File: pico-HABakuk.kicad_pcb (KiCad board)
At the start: 2 copper layers, 52 x 51.2 mm, 87 parts, among them J1 USB_B_Micro, J2 Ant+, J3 GPS Ant, J4 Ant-, J5 Solar, J6 Debug, J7 Super_Cap, Q1 BSS84, SW1 USB BOOT, SW2 RESET, U1 NCP1117-3.3_SOT223, U2 W25Q128JVS, U3 RP2040, U4 SPV1040T, U5 LM4040DBZ-3, U6 GP-02, U7 MAX809STRG, Y1 ABM8-272-T3

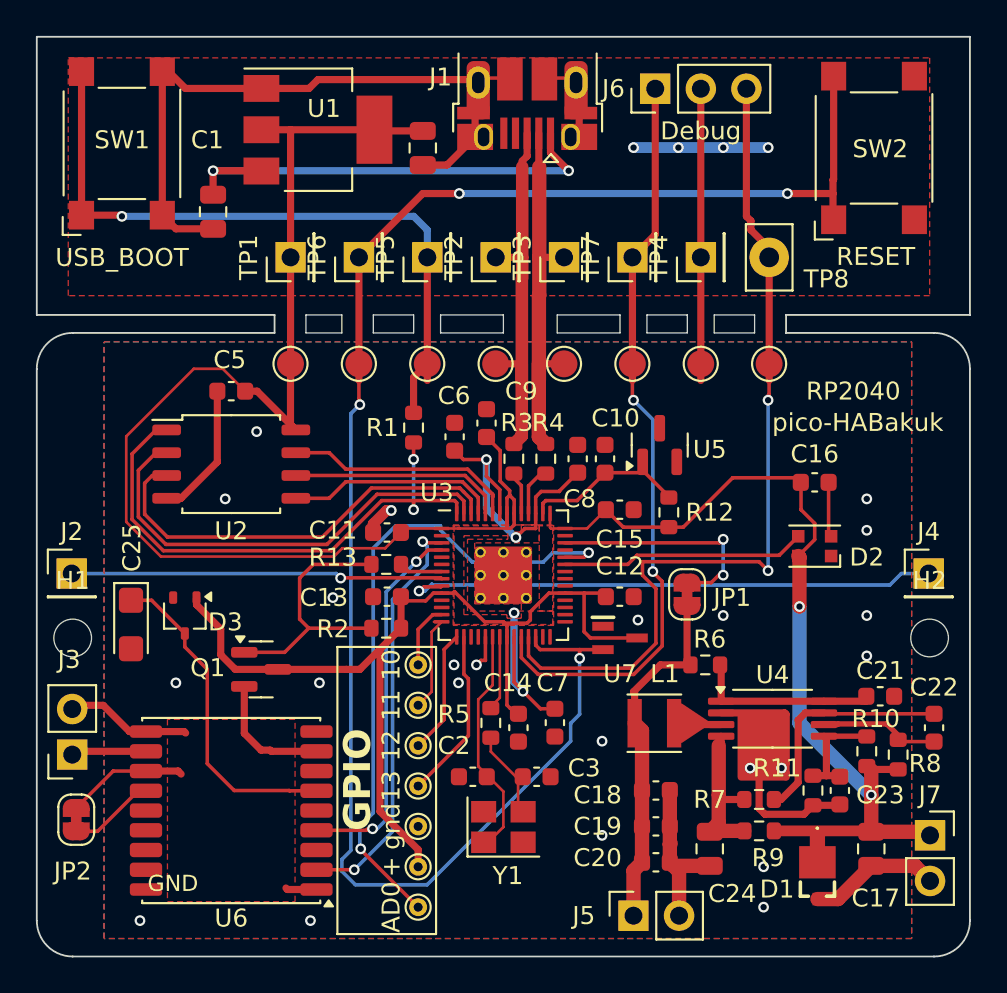
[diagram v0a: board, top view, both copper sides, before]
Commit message: Final board tuning and DRC debuging
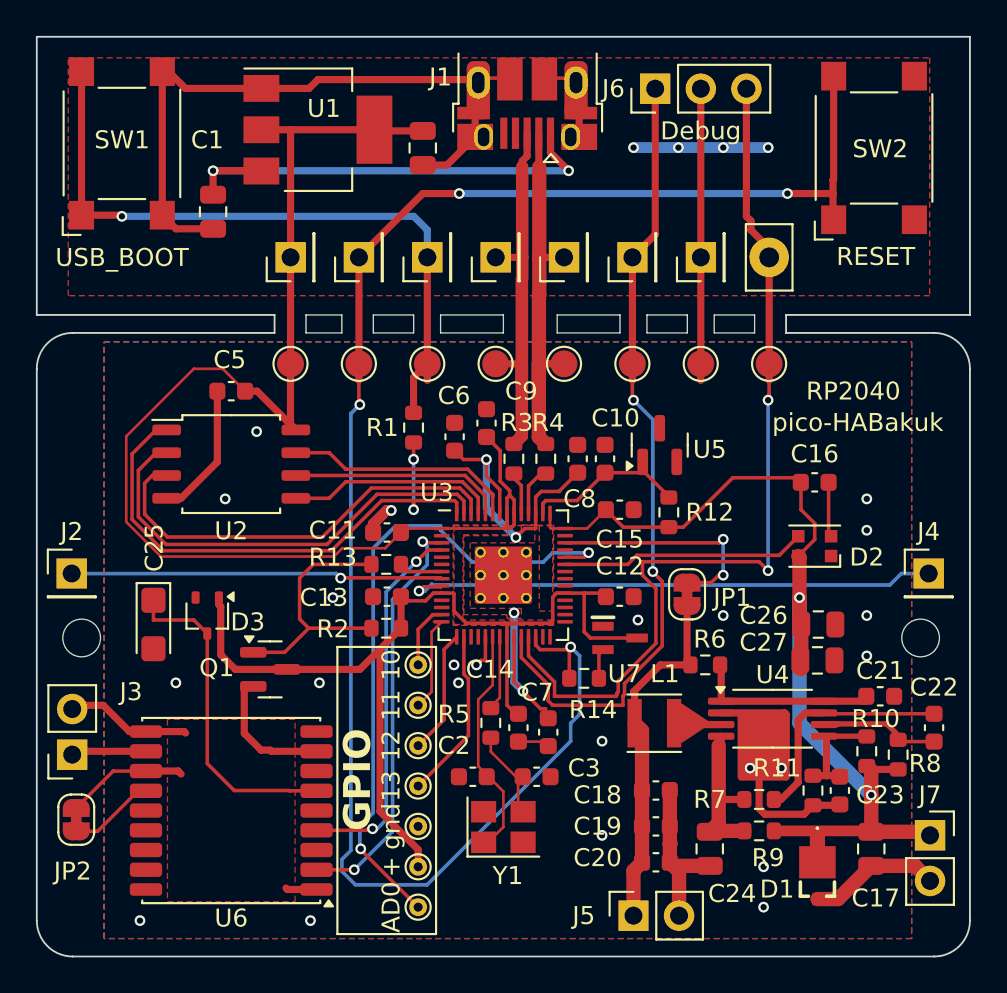
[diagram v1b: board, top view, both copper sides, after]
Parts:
- added C26: 10u, Capacitor_SMD:C_0805_2012Metric, F.Cu at (117.5, 102.8)
- added C27: 10u, Capacitor_SMD:C_0805_2012Metric, F.Cu at (117.5, 104.8)
- added R14: 2k2, Resistor_SMD:R_0603_1608Metric, F.Cu at (104.5, 105.8)
- TP10: value USB_D+ -> D+
- TP11: value USB_D- -> D-
- TP12: value GND -> gnd
- TP13: value USB_BOOT -> boot
- TP14: value Reset -> rst
- TP15: value SWCLK -> swclk
- TP16: value SWD -> swd
- TP9: value +3V3 -> +
- moved C25 1.25 mm to (80.5, 102.8)
- moved D3 1.25 mm to (83.5, 102.2)
- moved C7 0.65 mm to (102.5, 108.8)
- moved H1 0.50 mm to (76.5, 103.5)
- moved H2 0.50 mm to (123.2, 103.5)
- moved Q1 0.50 mm to (87.0, 105.2)
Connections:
- U7 pad 2: /RUN -> Net-(U7-~{RESET})
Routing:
- net +3V3: track 181.2 -> 185.8 mm
- net /SWCLK: track 43.3 -> 45.9 mm
- net /SWD: track 49.4 -> 51.6 mm
- net GND: track 126.8 -> 128.6 mm
- net Net-(U7-~{RESET}): track 0.00 -> 1.19 mm
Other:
- board text removed: "GND"
